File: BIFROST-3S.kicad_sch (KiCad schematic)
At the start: 6 parts, among them J1 B6B-XH-A_LF__SN_, J2 Conn_01x12, J3 B4B-XH-A_LF__SN_, J4 XT30PW-M

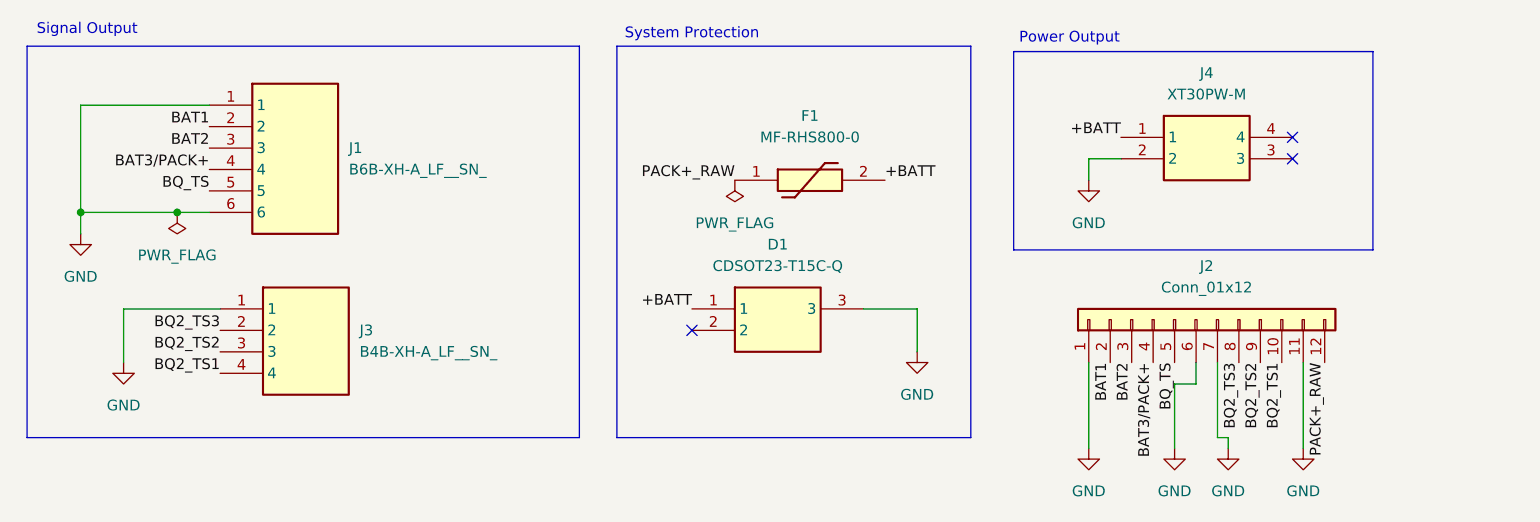
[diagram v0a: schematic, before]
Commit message: Layout 5.2
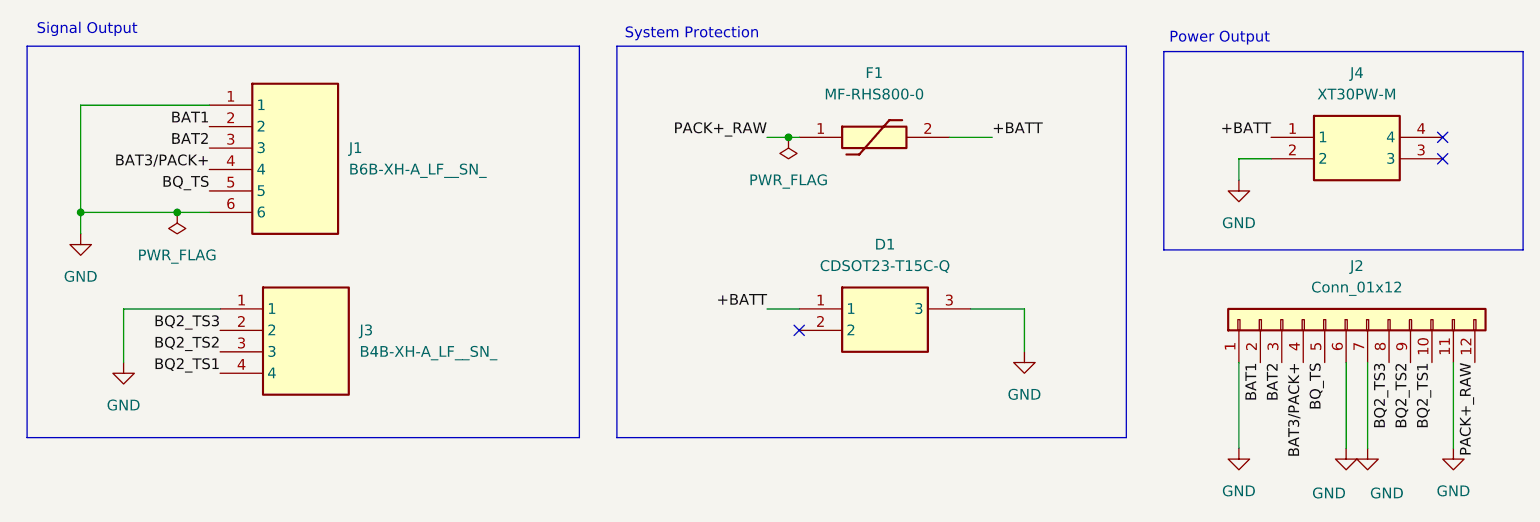
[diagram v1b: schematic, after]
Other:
- moved on the sheet: D1, J2, J4
